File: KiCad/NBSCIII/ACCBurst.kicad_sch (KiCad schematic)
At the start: 56 parts, among them Q901 BC337-25, Q902 BC337-25, Q903 BC337-25, Q910 BC337-25, Q911 BC337-25, Q912 BC337-25, U1 LM324N

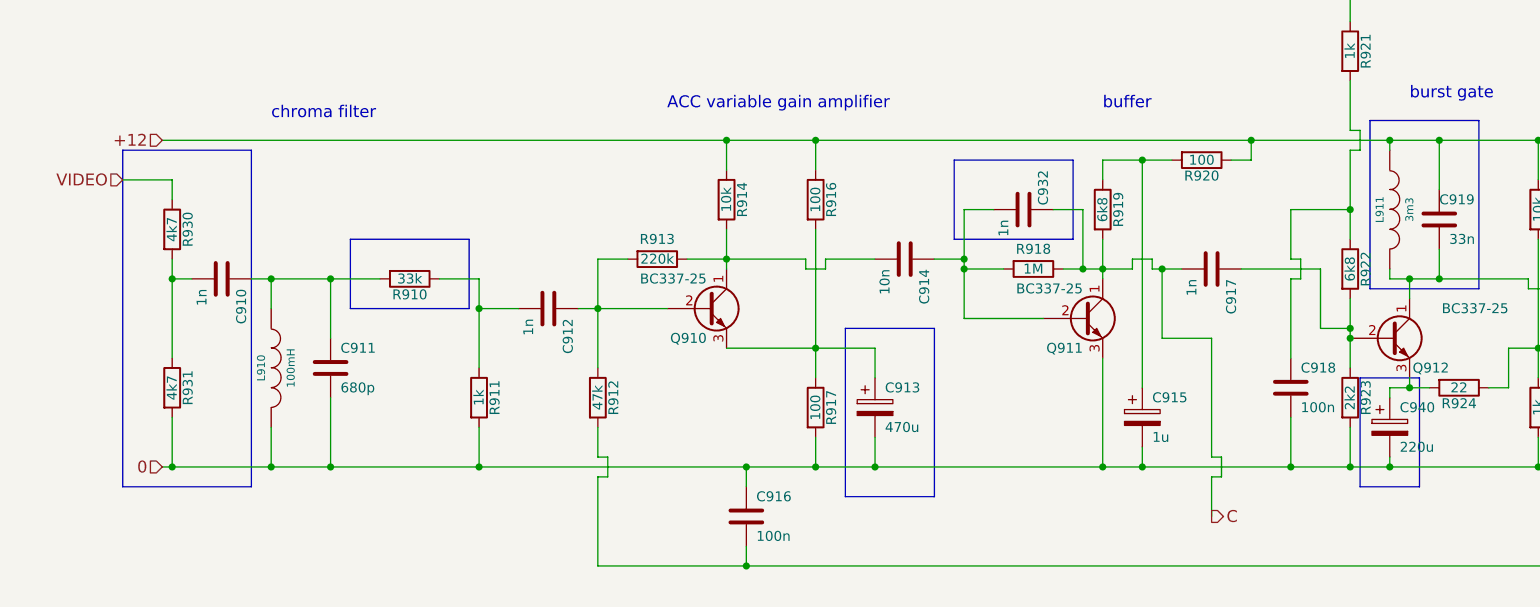
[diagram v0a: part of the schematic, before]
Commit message: unrescue Device:L_small
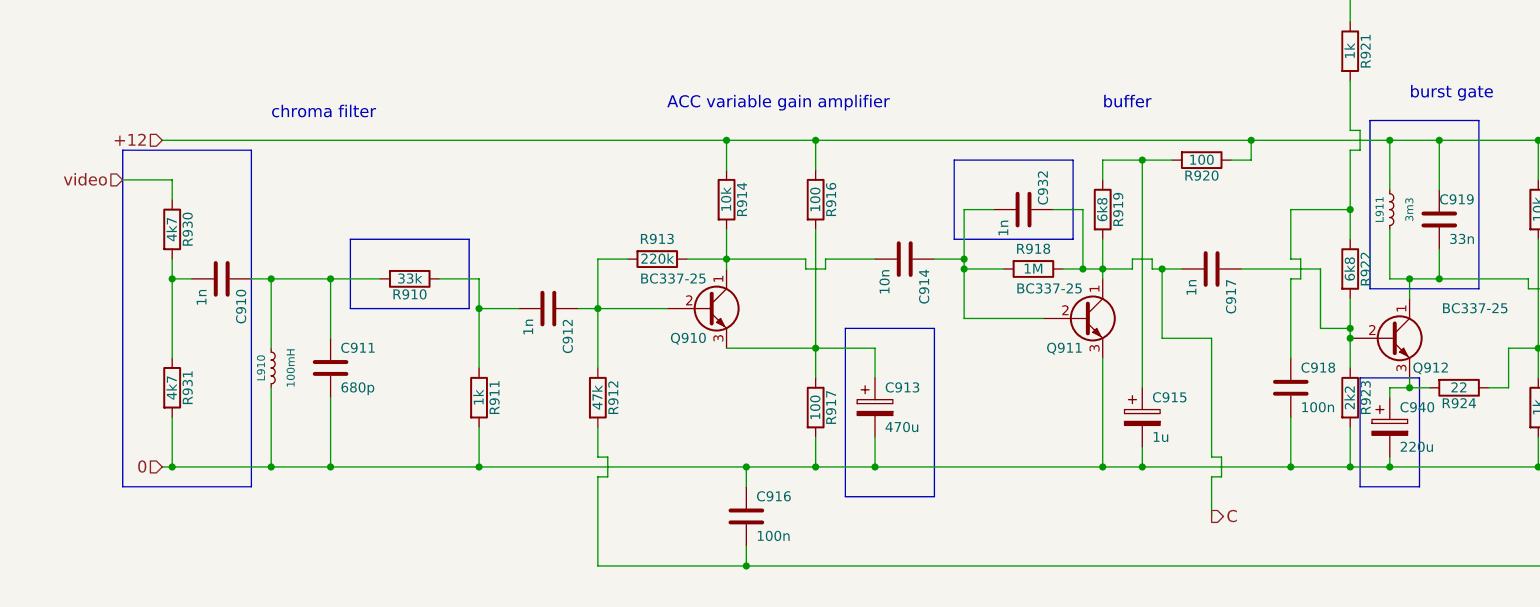
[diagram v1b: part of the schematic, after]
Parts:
- L910, L911: symbol NBSCIII-rescue:INDUCTOR -> Device:L_Small
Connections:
- net VIDEO renamed video
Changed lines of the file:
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@@
     (stroke (width 0) (type default) (color 0 0 0 0))
   )
-  (wire (pts (xy 41.91 109.22) (xy 41.91 105.41))
+  (wire (pts (xy 41.91 105.41) (xy 41.91 114.3))
     (stroke (width 0) (type default) (color 0 0 0 0))
   )
@@
     (stroke (width 0) (type default) (color 0 0 0 0))
   )
-  (wire (pts (xy 41.91 129.54) (xy 41.91 124.46))
+  (wire (pts (xy 41.91 119.38) (xy 41.91 129.54))
     (stroke (width 0) (type default) (color 0 0 0 0))
   )
@@
     (stroke (width 0) (type default) (color 0 0 0 0))
   )
-  (wire (pts (xy 185.42 87.63) (xy 185.42 88.9))
+  (wire (pts (xy 185.42 87.63) (xy 185.42 93.98))
     (stroke (width 0) (type default) (color 0 0 0 0))
   )
@@
     (stroke (width 0) (type default) (color 0 0 0 0))
   )
-  (wire (pts (xy 185.42 104.14) (xy 185.42 105.41))
+  (wire (pts (xy 185.42 99.06) (xy 185.42 105.41))
     (stroke (width 0) (type default) (color 0 0 0 0))
   )
@@
     (effects (font (size 1.524 1.524)) (justify right))
   )
-  (hierarchical_label "VIDEO" (shape input) (at 22.86 92.71 180)
+  (hierarchical_label "video" (shape input) (at 22.86 92.71 180)
     (effects (font (size 1.524 1.524)) (justify right))
   )
@@
     (pin "2")
   )
-  (symbol (lib_id "NBSCIII-rescue:INDUCTOR") (at 41.91 116.84 0) (unit 1)
+  (symbol (lib_id "Device:L_Small") (at 41.91 116.84 0) (unit 1)
     (in_bom yes) (on_board yes)
     (property "Reference" "L910" (id 0) (at 40.64 116.84 90)
@@
     (pin "2")
   )
-  (symbol (lib_id "NBSCIII-rescue:INDUCTOR") (at 185.42 96.52 0) (unit 1)
+  (symbol (lib_id "Device:L_Small") (at 185.42 96.52 0) (unit 1)
     (in_bom yes) (on_board yes)
     (property "Reference" "L911" (id 0) (at 184.15 96.52 90)
